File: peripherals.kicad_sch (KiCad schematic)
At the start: 7 parts, among them U5 BME280, U6 LSM303AGR, U7 MAX-M10S

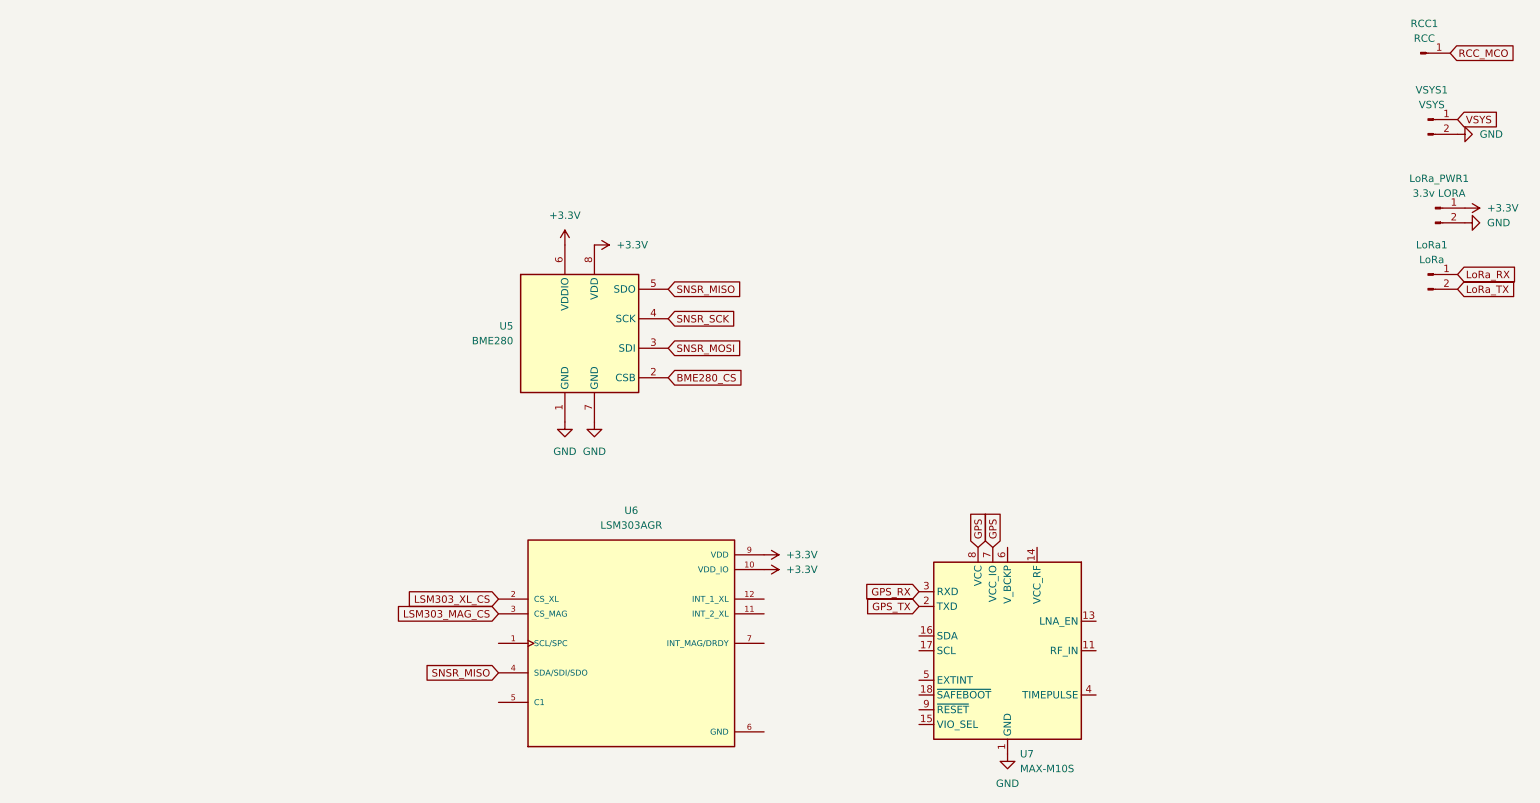
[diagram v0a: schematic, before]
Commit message: UPDATE U567
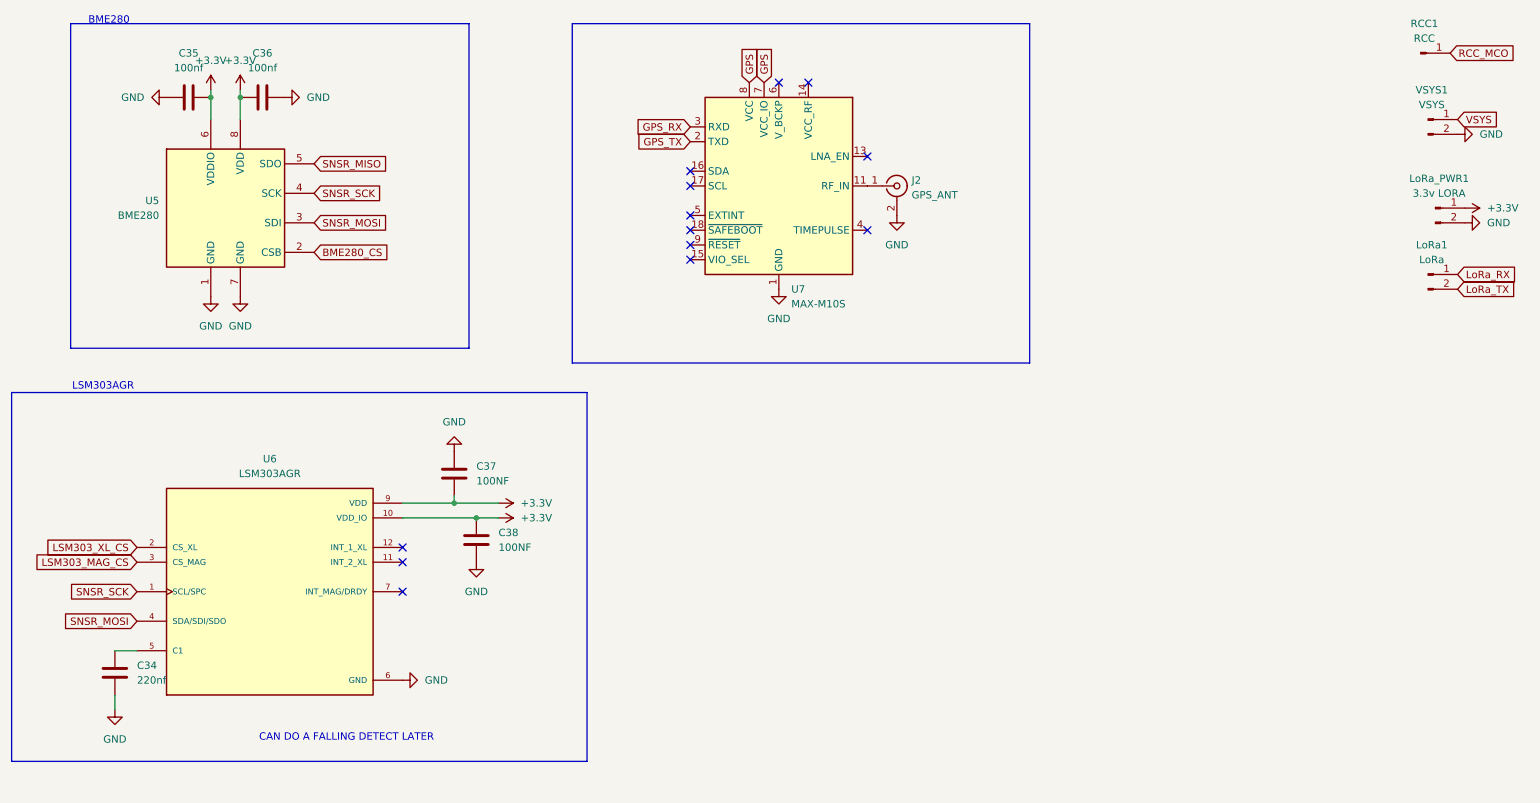
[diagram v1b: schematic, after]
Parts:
- added C34: 220nf, symbol Device:C
- added C35, C36: 100nf, symbol Device:C
- added C37, C38: 100NF, symbol Device:C
- added J2: GPS_ANT, symbol Connector:Conn_Coaxial
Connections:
- net +3.3V: now also C35.2, C36.1, C37.2, C38.1
- net GND: now also C34.1, C35.1, C36.2, C37.1, C38.2, J2.2 (Ext)
- net SNSR_MISO: no longer U6.4 (SDA/SDI/SDO)
- net SNSR_MOSI: now also U6.4 (SDA/SDI/SDO)
- net SNSR_SCK: now also U6.1 (SCL/SPC)
- net at U6.5 (C1): now also C34.2
- net at U7.11 (RF_IN): now also J2.1 (In)
- no-connect marks 0 -> 13
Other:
- note added: "BME280"
- note added: "CAN DO A FALLING DETECT LATER"
- note added: "LSM303AGR"
- moved on the sheet: U5, U6, U7
